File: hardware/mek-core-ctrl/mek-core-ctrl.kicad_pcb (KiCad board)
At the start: 2 copper layers, 150 x 100 mm, 16 parts, among them J1 24-26VAC, U1 LMR38020FDDAR, U2 AMS1117-3.3

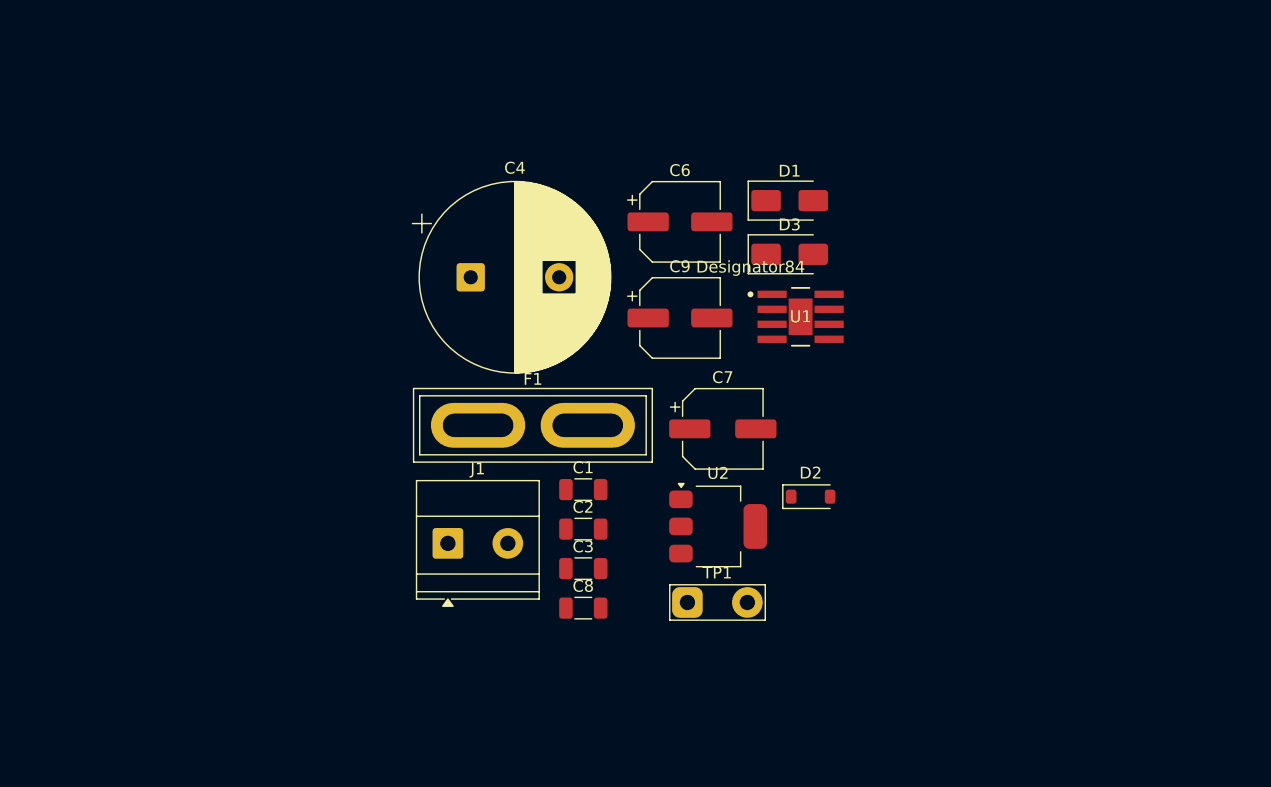
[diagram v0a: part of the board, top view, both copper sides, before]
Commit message: Creating mek-output-expander
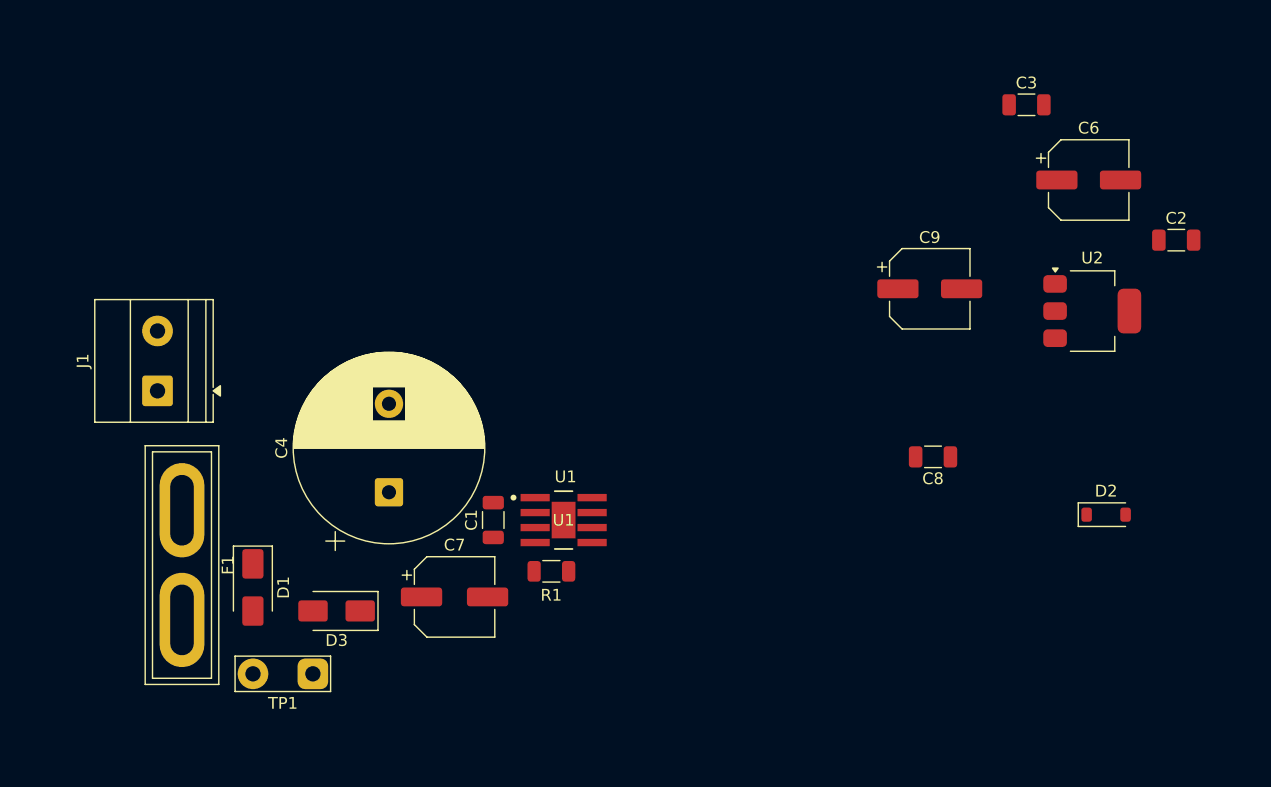
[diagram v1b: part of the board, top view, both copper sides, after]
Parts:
- added R1: 100k, Resistor_SMD:R_1206_3216Metric, F.Cu at (130.4, 112.6)
- moved D1 56.1 mm to (105.1, 114.0), turned to -90 degrees
- moved C2 55.9 mm to (183.4, 84.5)
- moved C3 54.4 mm to (170.7, 73.0)
- moved D3 48.9 mm to (112.2, 115.9), turned to 180 degrees
- moved U2 36.6 mm to (176.3, 90.5)
- moved C6 34.8 mm to (176.0, 79.4)
- moved TP1 32.3 mm to (110.2, 121.3), turned to 180 degrees
- moved C8 32.3 mm to (162.8, 102.9), turned to 180 degrees
- moved J1 27.8 mm to (97.0, 97.3), turned to 90 degrees
- moved C7 26.8 mm to (122.2, 114.8)
- moved U1 26.5 mm to (131.5, 108.2)
- moved F1 26.1 mm to (99.1, 107.4), turned to -90 degrees
- moved D2 25.1 mm to (177.4, 107.8)
- moved C9 21.3 mm to (162.5, 88.6)
- moved C4 19.5 mm to (116.7, 105.9), turned to 90 degrees
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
